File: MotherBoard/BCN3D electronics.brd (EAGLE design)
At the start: 70.5 x 95.8 mm, 87 parts, among them IC2 FT232RL, Q2 IRLS3034

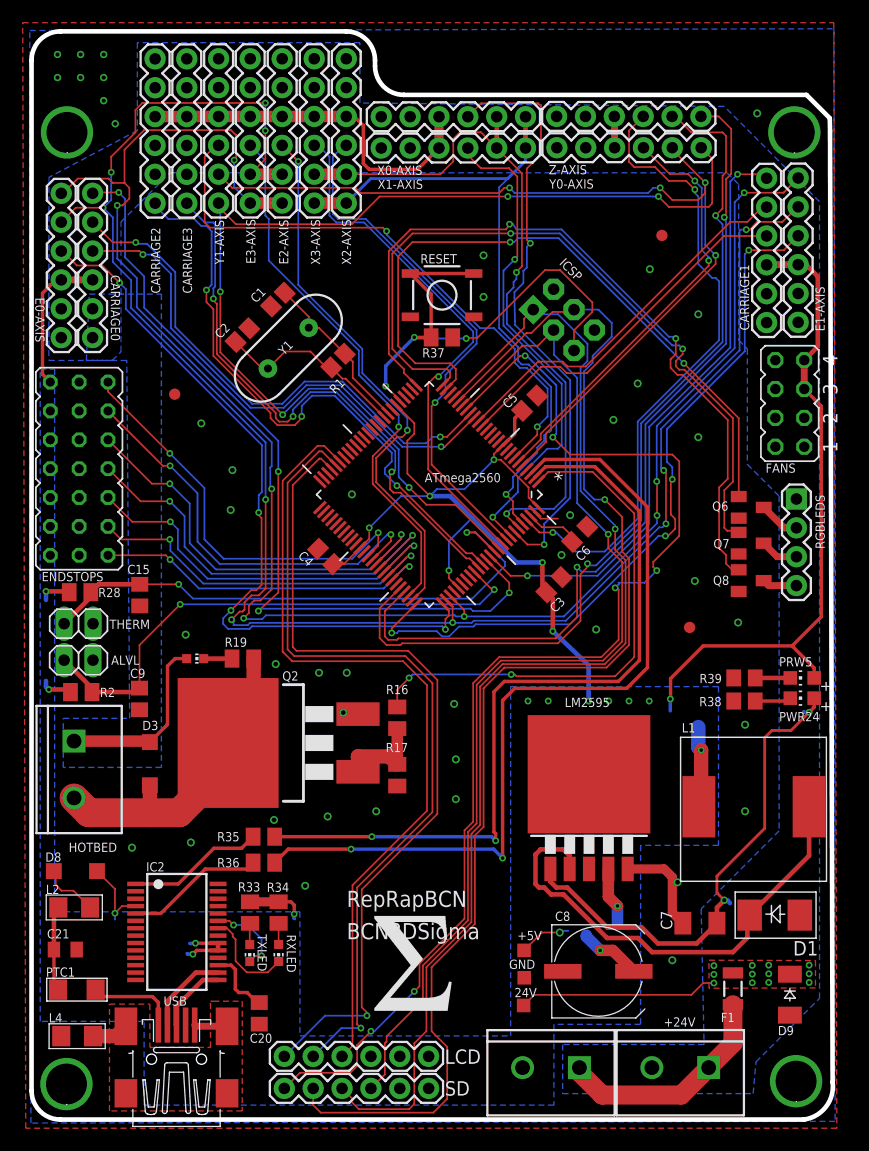
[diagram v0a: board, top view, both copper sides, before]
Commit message: New File Tree and Updates
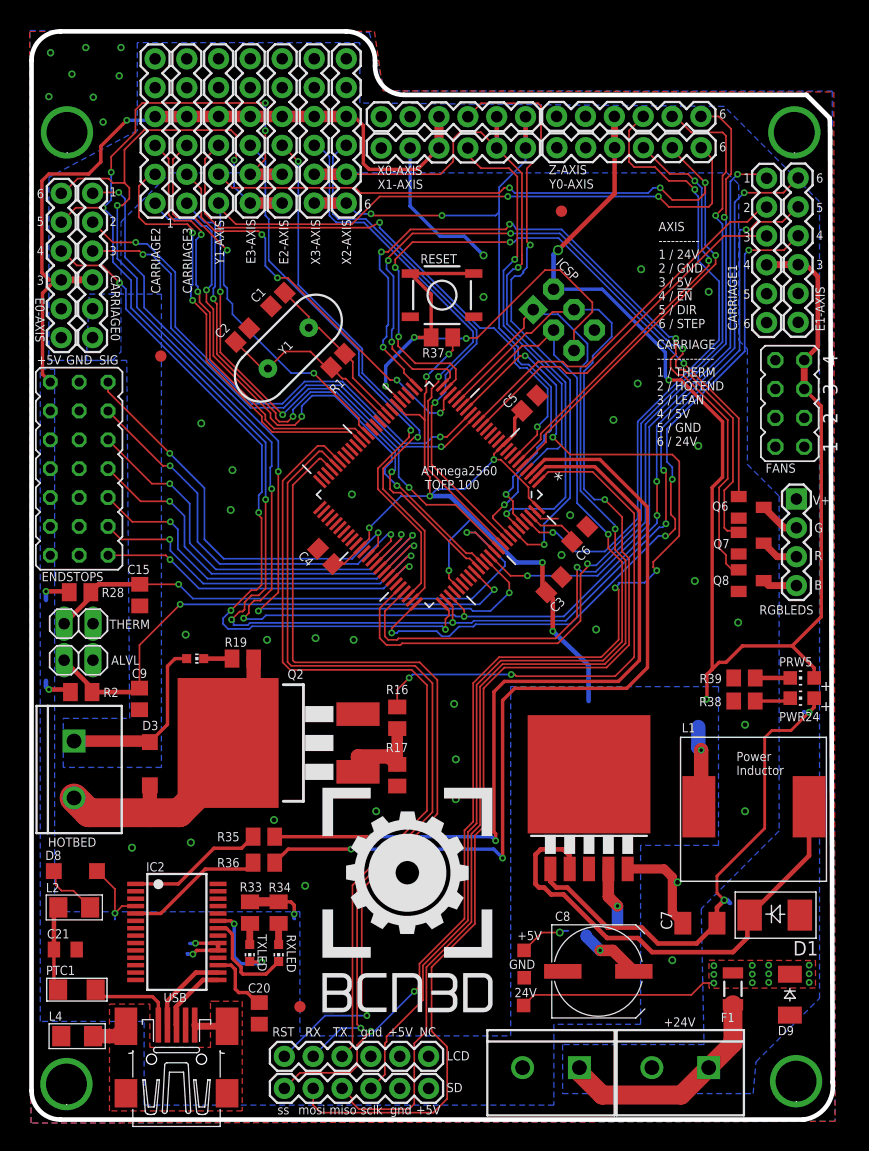
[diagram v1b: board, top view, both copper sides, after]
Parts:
- added DRILEGEND: (no value), drilegend:DRILEGEND
- U$5: device MarcEagleParts:SIGMA_LOGO -> MarcEagleParts:BCN3D_LOGO
- moved FID3 47.9 mm to (23.6, 9.93)
- moved LOGO1 21.3 mm to (16.1, 33.2)
- moved FID2 9.09 mm to (46.6, 79.9)
- moved U$5 3.98 mm to (25.6, 9.45)
- moved FID1 3.57 mm to (11.4, 67.2)
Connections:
- removed net 11111: ATMEGA2560.23
- removed net N$156: ATMEGA2560.38
- removed net N$157: ATMEGA2560.39
- removed net N$158: ATMEGA2560.40
- net GND: no longer U$1.GND
- net HOTEND2: now also ATMEGA2560.40
- net HOTEND3: now also ATMEGA2560.23
- net LFAN2: now also ATMEGA2560.39
- net LFAN3: now also ATMEGA2560.38
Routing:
- net +5V: track 226.6 -> 312.0 mm, vias 23 -> 22
- net LFAN2: track 0.00 -> 38.7 mm, vias 0 -> 2
- net HOTEND2: track 0.00 -> 38.7 mm, vias 0 -> 2
- net HOTEND3: track 0.00 -> 36.0 mm, vias 0 -> 4
- net LFAN3: track 0.00 -> 35.3 mm, vias 0 -> 2
- net GND: track 11.1 -> 24.5 mm, vias 43 -> 41
- net B-PWM: track 67.6 -> 69.0 mm, vias 2 -> 4
- net X-STEP: track 59.3 -> 58.2 mm, vias 1 -> 3
- net N$6: track 7.23 -> 8.26 mm
- net LCDRESET: track 74.2 -> 74.9 mm
- net LCDRX: track 73.0 -> 73.7 mm
- net LCDTX: track 71.6 -> 72.1 mm
- net R-PWM: track 66.3 -> 66.9 mm, vias 2 -> 4
- net X0-!EN: track 52.9 -> 53.4 mm
- net E3-!EN: track 48.3 -> 48.8 mm
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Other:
- board text added: "+"
- board text added: "+5V"
- board text added: "01-16"
- board text added: "01-20"
- board text added: "1"
- board text added: "2"
- board text added: "3"
- board text added: "4"
- board text added: "5"
- board text added: "6"
- board text added: "ATmega2560 TQFP 100"
- board text added: "AXIS ---------- 1 / 24V 2 / GND 3 / 5V 4 / !EN 5 / DIR 6 / STEP"
- board text added: "B"
- board text added: "BCN3D Electronics Designed in Barcelona ---------------------------------- MotherBoard - Nov 2014 Marc Cobler - REV_A"
- board text added: "CARRIAGE -------------- 1 / THERM 2 / HOTEND 3 / LFAN 4 / 5V 5 / GND 6 / 24V"
- board text added: "G"
- board text added: "GND"
- board text added: "LAYER-STACK"
- board text added: "NC"
- board text added: "Power Inductor"
- board text added: "R"
- board text added: "RST"
- board text added: "RX"
- board text added: "SIG"
- board text added: "TX"
- board text added: "V+"
- board text added: "gnd"
- board text added: "miso"
- board text added: "mosi"
- board text added: "sclk"
- board text added: "ss"
- board text removed: "ATmega2560"
- board text removed: "BCNelectronics - RepRapBCN Designed in Barcelona ---------------------------------- Sigma MotherBoard Marc Cobler - REV_A Nov 2014"
- board text removed: "RepRapBCN BCN3DSigma"

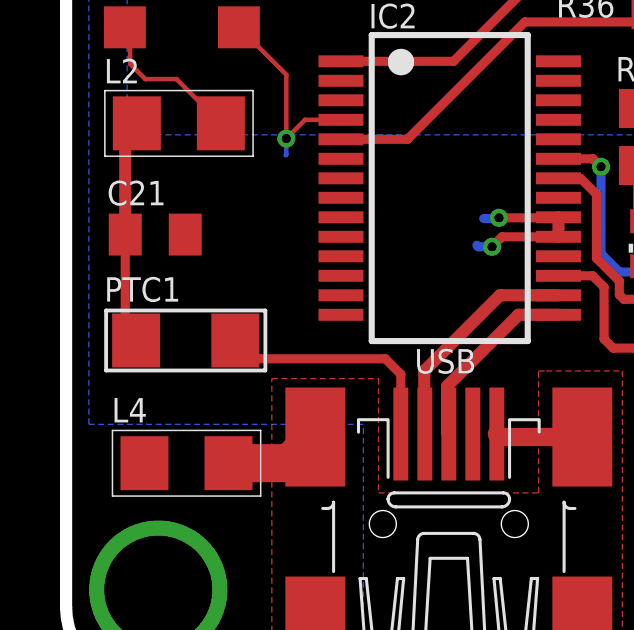
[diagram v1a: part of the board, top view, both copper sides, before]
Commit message: Updates!
Rev_A Ready and firsts prototypes
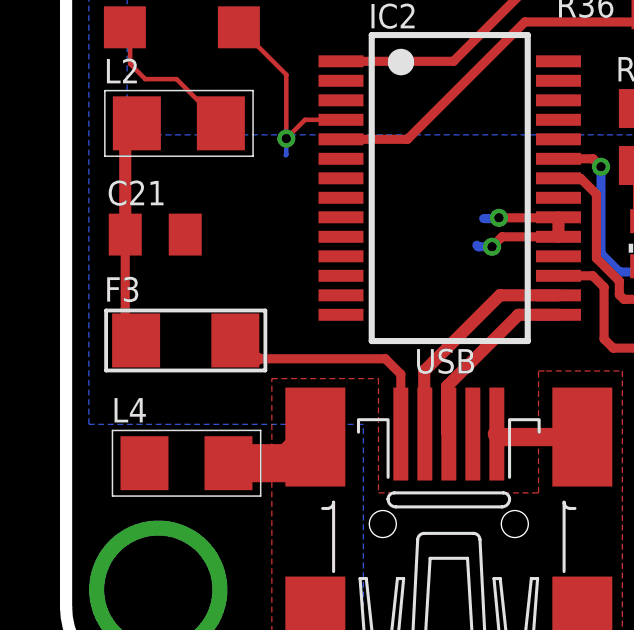
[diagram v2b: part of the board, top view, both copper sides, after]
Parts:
- F1: value PTCSMD -> IN_PTC
- renumbered PTC1 to F3
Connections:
- net GND: now also U$1.GND
